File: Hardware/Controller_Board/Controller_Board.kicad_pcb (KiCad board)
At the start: 2 copper layers, 155 parts, among them Q1 DMN2400UFB-7, SW1 Reset, U1 TPS82084, U10 FT232H, U11 93LC56B, U2 LT8645S, U3 TPS82084, U4 TPS82084, U5 XT30, U6 XC7A35T-CPG236, U7 IS25LP256D, U8 FT232H, U9 93LC56B, Y1 12MHz, Y2 12MHz

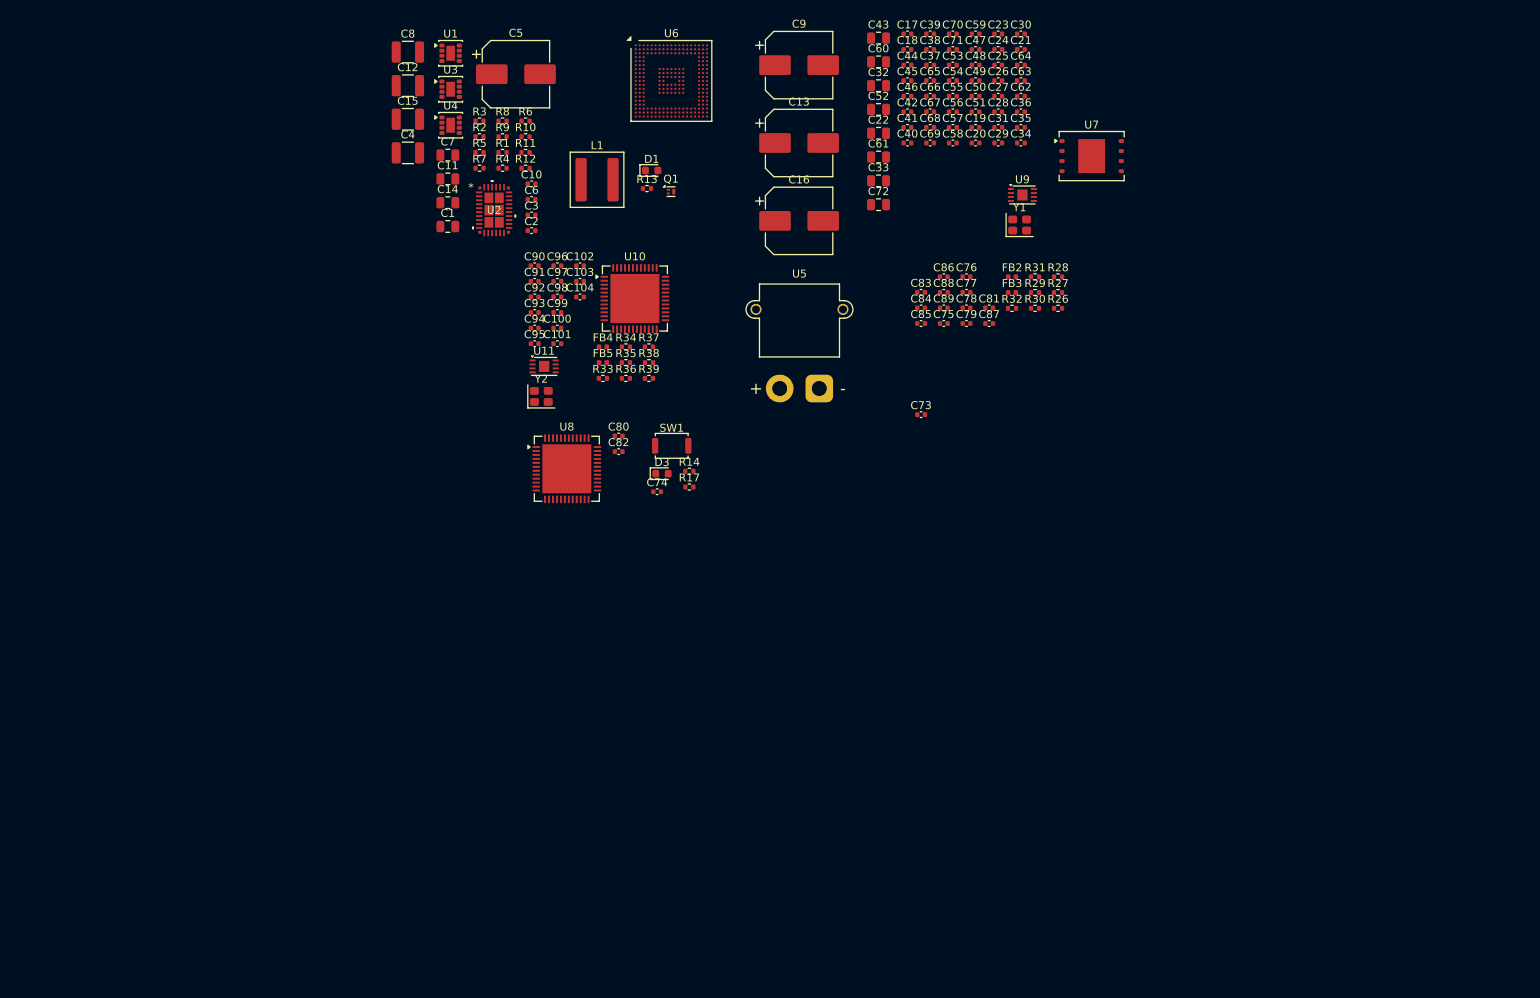
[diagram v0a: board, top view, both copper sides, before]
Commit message: Updated the schematic design - Fix the XC7A35T-CPG236 outline issue
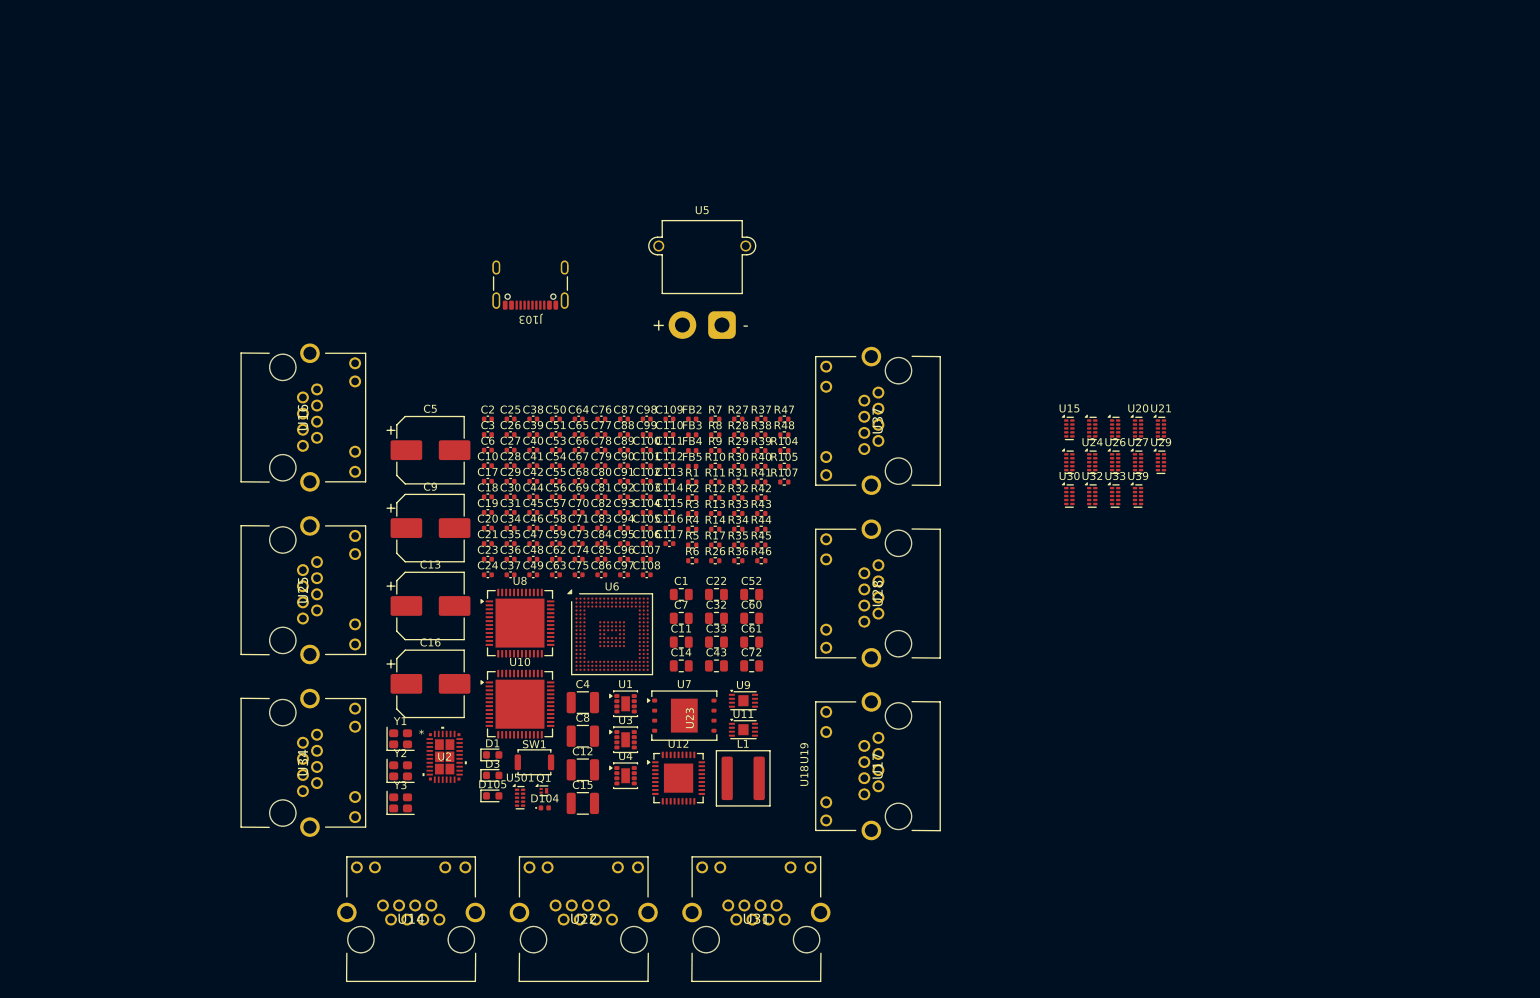
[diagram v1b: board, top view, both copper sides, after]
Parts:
- added C105: 10p, Capacitor_SMD:C_0402_1005Metric, F.Cu at (132.7, 94.0)
- added C106: 10p, Capacitor_SMD:C_0402_1005Metric, F.Cu at (132.7, 95.9)
- added C107: 4u7, Capacitor_SMD:C_0402_1005Metric, F.Cu at (132.7, 97.9)
- added C108: 100n, Capacitor_SMD:C_0402_1005Metric, F.Cu at (132.7, 99.9)
- added C109: 100n, Capacitor_SMD:C_0402_1005Metric, F.Cu at (135.6, 80.2)
- added C110: 100n, Capacitor_SMD:C_0402_1005Metric, F.Cu at (135.6, 82.1)
- added C111: 100n, Capacitor_SMD:C_0402_1005Metric, F.Cu at (135.6, 84.1)
- added C112: 100n, Capacitor_SMD:C_0402_1005Metric, F.Cu at (135.6, 86.1)
- added C113: 100n, Capacitor_SMD:C_0402_1005Metric, F.Cu at (135.6, 88.0)
- added C114: 10n, Capacitor_SMD:C_0402_1005Metric, F.Cu at (135.6, 90.0)
- added C115: 100n, Capacitor_SMD:C_0402_1005Metric, F.Cu at (135.6, 92.0)
- added C116: 10n, Capacitor_SMD:C_0402_1005Metric, F.Cu at (135.6, 94.0)
- added C117: 100n, Capacitor_SMD:C_0402_1005Metric, F.Cu at (135.6, 95.9)
- added D104: TVS, Diode_SMD:D_0402_1005Metric, F.Cu at (119.8, 129.3)
- added D105: LED, LED_SMD:LED_0603_1608Metric, F.Cu at (113.2, 127.8)
- added J103: USB_C_USB2.0, Connector_USB:USB_C_Receptacle_GCT_USB4105-xx-A_16P_TopMnt_Horizontal, F.Cu at (118.0, 62.1)
- added R104: 5k1, Resistor_SMD:R_0402_1005Metric, F.Cu at (150.1, 84.2)
- added R105: 5k1, Resistor_SMD:R_0402_1005Metric, F.Cu at (150.1, 86.1)
- added R107: 1k, Resistor_SMD:R_0402_1005Metric, F.Cu at (150.1, 88.1)
- added R40: 22R, Resistor_SMD:R_0402_1005Metric, F.Cu at (147.2, 86.1)
- added R41: 12k, Resistor_SMD:R_0402_1005Metric, F.Cu at (147.2, 88.1)
- added R42: 100k, Resistor_SMD:R_0402_1005Metric, F.Cu at (147.2, 90.1)
- added R43: 100k, Resistor_SMD:R_0402_1005Metric, F.Cu at (147.2, 92.1)
- added R44: 100k, Resistor_SMD:R_0402_1005Metric, F.Cu at (147.2, 94.1)
- added R45: 100k, Resistor_SMD:R_0402_1005Metric, F.Cu at (147.2, 96.1)
- added R46: 100k, Resistor_SMD:R_0402_1005Metric, F.Cu at (147.2, 98.1)
- added R47: 100k, Resistor_SMD:R_0402_1005Metric, F.Cu at (150.1, 80.2)
- added R48: 1k, Resistor_SMD:R_0402_1005Metric, F.Cu at (150.1, 82.2)
- added U12: USB2512B, Package_DFN_QFN:QFN-36-1EP_6x6mm_P0.5mm_EP3.7x3.7mm, F.Cu at (136.7, 125.6)
- added U14: RJ45, Custom_VoxLink_Footprints:TE_RJ45, F.Cu at (102.9, 146.0)
- added U15: TPD4E02B04, Package_SON:USON-10_2.5x1.0mm_P0.5mm, F.Cu at (186.1, 81.3)
- added U16: RJ45, Custom_VoxLink_Footprints:TE_RJ45, F.Cu at (86.7, 80.0)
- added U17: RJ45, Custom_VoxLink_Footprints:TE_RJ45, F.Cu at (164.5, 124.1)
- added U18: TPD4E02B04, Package_SON:USON-10_2.5x1.0mm_P0.5mm, F.Cu at (189.0, 81.3)
- added U19: TPD4E02B04, Package_SON:USON-10_2.5x1.0mm_P0.5mm, F.Cu at (191.9, 81.3)
- added U20: TPD4E02B04, Package_SON:USON-10_2.5x1.0mm_P0.5mm, F.Cu at (194.8, 81.3)
- added U21: TPD4E02B04, Package_SON:USON-10_2.5x1.0mm_P0.5mm, F.Cu at (197.7, 81.3)
- added U22: RJ45, Custom_VoxLink_Footprints:TE_RJ45, F.Cu at (124.7, 146.0)
- added U23: TPD4E02B04, Package_SON:USON-10_2.5x1.0mm_P0.5mm, F.Cu at (186.1, 85.6)
- added U24: TPD4E02B04, Package_SON:USON-10_2.5x1.0mm_P0.5mm, F.Cu at (189.0, 85.6)
- added U25: RJ45, Custom_VoxLink_Footprints:TE_RJ45, F.Cu at (86.7, 101.8)
- added U26: TPD4E02B04, Package_SON:USON-10_2.5x1.0mm_P0.5mm, F.Cu at (191.9, 85.6)
- added U27: TPD4E02B04, Package_SON:USON-10_2.5x1.0mm_P0.5mm, F.Cu at (194.8, 85.6)
- added U28: RJ45, Custom_VoxLink_Footprints:TE_RJ45, F.Cu at (164.5, 102.2)
- added U29: TPD4E02B04, Package_SON:USON-10_2.5x1.0mm_P0.5mm, F.Cu at (197.7, 85.6)
- added U30: TPD4E02B04, Package_SON:USON-10_2.5x1.0mm_P0.5mm, F.Cu at (186.1, 89.9)
- added U31: RJ45, Custom_VoxLink_Footprints:TE_RJ45, F.Cu at (146.6, 146.0)
- added U32: TPD4E02B04, Package_SON:USON-10_2.5x1.0mm_P0.5mm, F.Cu at (189.0, 89.9)
- added U33: TPD4E02B04, Package_SON:USON-10_2.5x1.0mm_P0.5mm, F.Cu at (191.9, 89.9)
- added U34: RJ45, Custom_VoxLink_Footprints:TE_RJ45, F.Cu at (86.7, 123.6)
- added U37: RJ45, Custom_VoxLink_Footprints:TE_RJ45, F.Cu at (164.5, 80.4)
- added U39: TPD4E02B04, Package_SON:USON-10_2.5x1.0mm_P0.5mm, F.Cu at (194.8, 89.9)
- added U501: TPD4E02B04, Package_SON:USON-10_2.5x1.0mm_P0.5mm, F.Cu at (116.7, 128.0)
- added Y3: 24MHz, Crystal:Crystal_SMD_2520-4Pin_2.5x2.0mm, F.Cu at (101.5, 128.7)
- moved Y1 101.7 mm to (101.5, 120.6)
- moved C23 92.6 mm to (112.6, 97.9)
- moved C24 92.6 mm to (112.6, 99.9)
- moved C21 91.9 mm to (112.6, 95.9)
- moved C15 89.3 mm to (124.6, 128.8)
- moved C12 89.3 mm to (124.6, 124.5)
- moved C8 89.3 mm to (124.6, 120.3)
- moved U7 87.5 mm to (137.4, 117.7)
- moved C30 87.1 mm to (115.5, 90.0)
- moved C36 85.8 mm to (115.5, 97.9)
- moved C63 85.8 mm to (121.2, 99.9)
- moved U1 85.2 mm to (130.0, 116.2)
- moved U3 85.2 mm to (130.0, 120.7)
- moved U4 85.2 mm to (130.0, 125.3)
- moved C47 83.9 mm to (118.3, 95.9)
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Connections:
- U10 pad 6: FTDI_USB_D- -> SERIAL_D-
- U10 pad 7: FTDI_USB_D+ -> SERIAL_D+
- U8 pad 6: FTDI_USB_D- -> JTAG_D-
- U8 pad 7: FTDI_USB_D+ -> JTAG_D+

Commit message: Finished schematic design - preparation for review
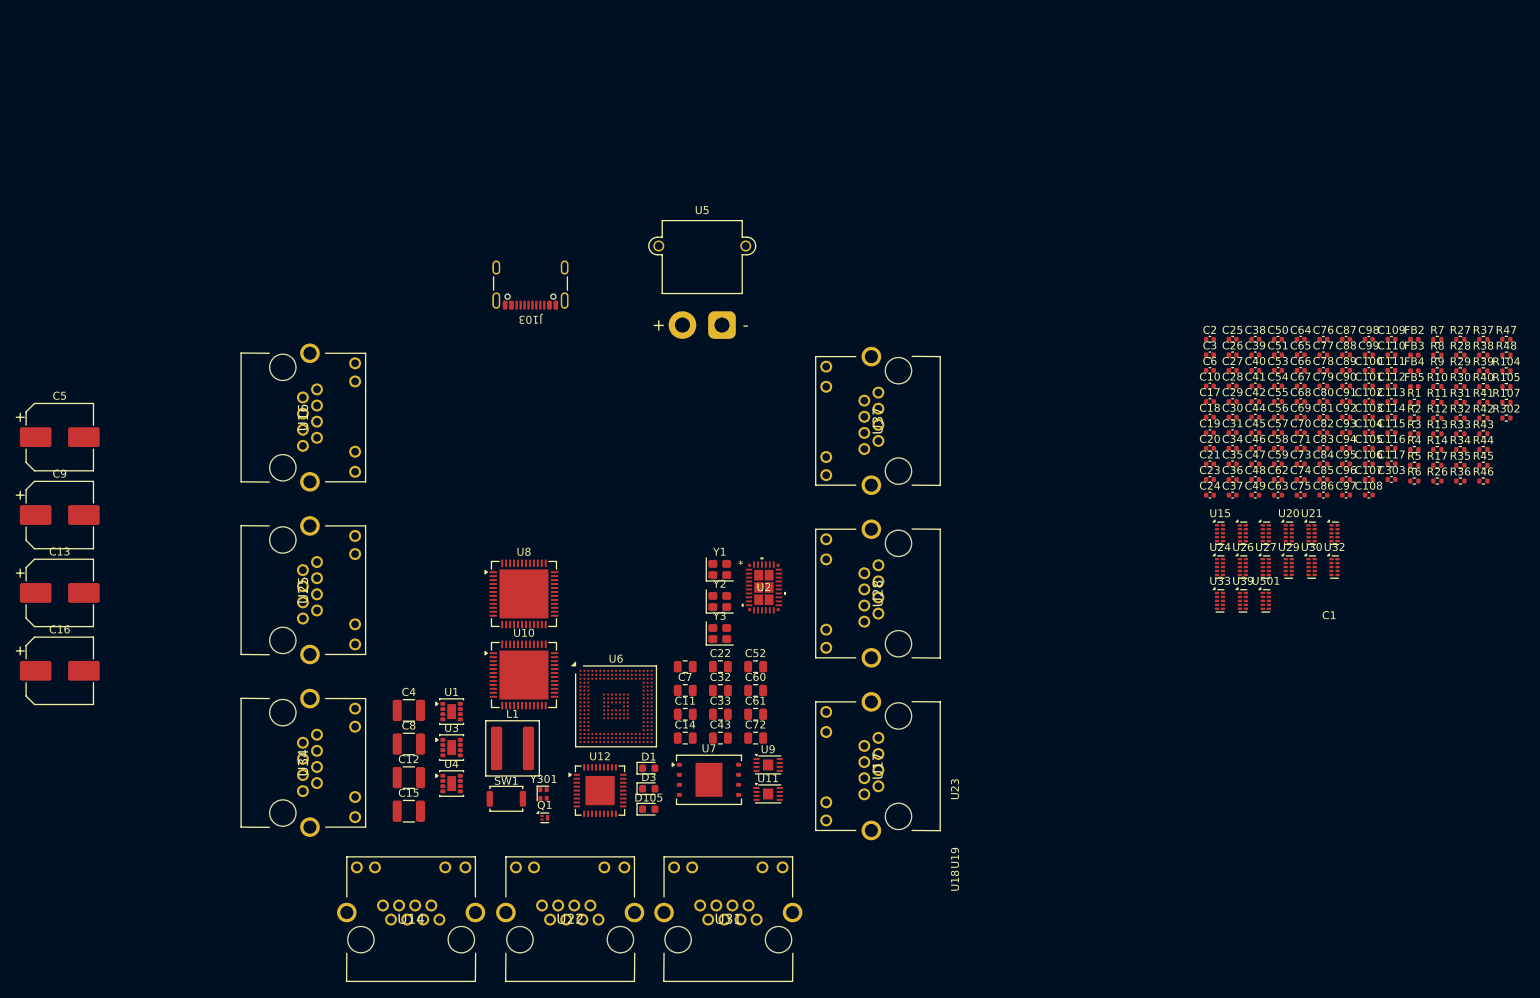
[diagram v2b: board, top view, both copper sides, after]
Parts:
- removed D104: TVS, Diode_SMD:D_0402_1005Metric
- added C303: 100n, Capacitor_SMD:C_0402_1005Metric, F.Cu at (226.9, 87.8)
- added R302: 22R, Resistor_SMD:R_0402_1005Metric, F.Cu at (241.4, 80.0)
- added Y301: 12MHz, Oscillator:Oscillator_SMD_Abracon_ASCO-4Pin_1.6x1.2mm, F.Cu at (119.6, 127.6)
- moved U501 97.5 mm to (211.0, 103.2)
- moved R27 91.9 mm to (235.6, 70.1)
- moved R28 91.9 mm to (235.6, 72.1)
- moved R29 91.9 mm to (235.6, 74.1)
- moved R30 91.9 mm to (235.6, 76.1)
- moved R31 91.9 mm to (235.6, 78.0)
- moved R32 91.9 mm to (235.6, 80.0)
- moved R33 91.9 mm to (235.6, 82.0)
- moved R34 91.9 mm to (235.6, 84.0)
- moved R35 91.9 mm to (235.6, 86.0)
- moved R36 91.9 mm to (235.6, 88.0)
- moved R37 91.9 mm to (238.5, 70.1)
- moved R38 91.9 mm to (238.5, 72.1)
- moved R39 91.9 mm to (238.5, 74.1)
- moved R40 91.9 mm to (238.5, 76.1)
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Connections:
- U14 pad 1: Net-(U14-RX) -> /Connectivity/P1_RX_P
- U14 pad 2: Net-(U14-~{RX}) -> /Connectivity/P1_RX_N
- U14 pad 4: Net-(U14-CLK) -> /Connectivity/P1_CLK_P
- U14 pad 5: Net-(U14-~{CLK}) -> /Connectivity/P1_CLK_N
- U14 pad 7: Net-(U14-~{TX}) -> /Connectivity/P1_TX_N
- U14 pad 8: Net-(U14-TX) -> /Connectivity/P1_TX_P
- U15 pad 1: Net-(U14-RX) -> /Connectivity/P1_RX_P
- U15 pad 10: unconnected-(U15-NC-Pad10) -> /Connectivity/P1_RX_P
- U15 pad 2: Net-(U14-~{RX}) -> /Connectivity/P1_RX_N
- U15 pad 4: Net-(U16-CLK) -> /Connectivity/P2_CLK_P
- U15 pad 5: Net-(U16-~{CLK}) -> /Connectivity/P2_CLK_N
- U15 pad 6: unconnected-(U15-NC-Pad6) -> /Connectivity/P2_CLK_N
- U15 pad 7: unconnected-(U15-NC-Pad7) -> /Connectivity/P2_CLK_P
- U15 pad 9: unconnected-(U15-NC-Pad9) -> /Connectivity/P1_RX_N
- U16 pad 1: Net-(U16-RX) -> /Connectivity/P2_RX_P
- U16 pad 2: Net-(U16-~{RX}) -> /Connectivity/P2_RX_N
- U16 pad 4: Net-(U16-CLK) -> /Connectivity/P2_CLK_P
- U16 pad 5: Net-(U16-~{CLK}) -> /Connectivity/P2_CLK_N
- U16 pad 7: Net-(U16-~{TX}) -> /Connectivity/P2_TX_N
- U16 pad 8: Net-(U16-TX) -> /Connectivity/P2_TX_P
- U17 pad 1: Net-(U17-RX) -> /Connectivity/P3_RX_P
- U17 pad 2: Net-(U17-~{RX}) -> /Connectivity/P3_RX_N
- U17 pad 4: Net-(U17-CLK) -> /Connectivity/P3_CLK_P
- U17 pad 5: Net-(U17-~{CLK}) -> /Connectivity/P3_CLK_N
- U17 pad 7: Net-(U17-~{TX}) -> /Connectivity/P3_TX_N
- U17 pad 8: Net-(U17-TX) -> /Connectivity/P3_TX_P
- U18 pad 1: Net-(U17-~{TX}) -> /Connectivity/P3_TX_N
- U18 pad 10: unconnected-(U18-NC-Pad10) -> /Connectivity/P3_TX_N
- U18 pad 2: Net-(U17-TX) -> /Connectivity/P3_TX_P
- U18 pad 4: Net-(U17-~{CLK}) -> /Connectivity/P3_CLK_N
- U18 pad 5: Net-(U17-CLK) -> /Connectivity/P3_CLK_P
- U18 pad 6: unconnected-(U18-NC-Pad6) -> /Connectivity/P3_CLK_P
- U18 pad 7: unconnected-(U18-NC-Pad7) -> /Connectivity/P3_CLK_N
- U18 pad 9: unconnected-(U18-NC-Pad9) -> /Connectivity/P3_TX_P
- U19 pad 4: Net-(U17-~{RX}) -> /Connectivity/P3_RX_N
- U19 pad 5: Net-(U17-RX) -> /Connectivity/P3_RX_P
- U19 pad 6: unconnected-(U19-NC-Pad6) -> /Connectivity/P3_RX_P
- U19 pad 7: unconnected-(U19-NC-Pad7) -> /Connectivity/P3_RX_N
- U20 pad 1: Net-(U16-~{RX}) -> /Connectivity/P2_RX_N
- U20 pad 10: unconnected-(U20-NC-Pad10) -> /Connectivity/P2_RX_N
- U20 pad 2: Net-(U16-RX) -> /Connectivity/P2_RX_P
- U20 pad 4: Net-(U16-~{TX}) -> /Connectivity/P2_TX_N
- U20 pad 5: Net-(U16-TX) -> /Connectivity/P2_TX_P
- U20 pad 6: unconnected-(U20-NC-Pad6) -> /Connectivity/P2_TX_P
- U20 pad 7: unconnected-(U20-NC-Pad7) -> /Connectivity/P2_TX_N
- U20 pad 9: unconnected-(U20-NC-Pad9) -> /Connectivity/P2_RX_P
- U21 pad 1: Net-(U37-~{TX}) -> /Connectivity/P9_TX_N
- U21 pad 10: unconnected-(U21-NC-Pad10) -> /Connectivity/P9_TX_N
- U21 pad 2: Net-(U37-TX) -> /Connectivity/P9_TX_P
- U21 pad 4: Net-(U37-~{CLK}) -> /Connectivity/P9_CLK_N
- U21 pad 5: Net-(U37-CLK) -> /Connectivity/P9_CLK_P
- U21 pad 6: unconnected-(U21-NC-Pad6) -> /Connectivity/P9_CLK_P
- U21 pad 7: unconnected-(U21-NC-Pad7) -> /Connectivity/P9_CLK_N
- U21 pad 9: unconnected-(U21-NC-Pad9) -> /Connectivity/P9_TX_P
- U22 pad 1: Net-(U22-RX) -> /Connectivity/P4_RX_P
- U22 pad 2: Net-(U22-~{RX}) -> /Connectivity/P4_RX_N
- U22 pad 4: Net-(U22-CLK) -> /Connectivity/P4_CLK_P
- U22 pad 5: Net-(U22-~{CLK}) -> /Connectivity/P4_CLK_N
- U22 pad 7: Net-(U22-~{TX}) -> /Connectivity/P4_TX_N
- U22 pad 8: Net-(U22-TX) -> /Connectivity/P4_TX_P
- U23 pad 1: Net-(U22-~{TX}) -> /Connectivity/P4_TX_N
- U23 pad 10: unconnected-(U23-NC-Pad10) -> /Connectivity/P4_TX_N
- U23 pad 2: Net-(U22-TX) -> /Connectivity/P4_TX_P
- U23 pad 4: Net-(U22-~{CLK}) -> /Connectivity/P4_CLK_N
- U23 pad 5: Net-(U22-CLK) -> /Connectivity/P4_CLK_P
- U23 pad 6: unconnected-(U23-NC-Pad6) -> /Connectivity/P4_CLK_P
- U23 pad 7: unconnected-(U23-NC-Pad7) -> /Connectivity/P4_CLK_N
- U23 pad 9: unconnected-(U23-NC-Pad9) -> /Connectivity/P4_TX_P
- U24 pad 1: Net-(U25-~{RX}) -> /Connectivity/P5_RX_N
- U24 pad 10: unconnected-(U24-NC-Pad10) -> /Connectivity/P5_RX_N
- U24 pad 2: Net-(U25-RX) -> /Connectivity/P5_RX_P
- U24 pad 4: Net-(U25-~{TX}) -> /Connectivity/P5_TX_N
- U24 pad 5: Net-(U25-TX) -> /Connectivity/P5_TX_P
- U24 pad 6: unconnected-(U24-NC-Pad6) -> /Connectivity/P5_TX_P
- U24 pad 7: unconnected-(U24-NC-Pad7) -> /Connectivity/P5_TX_N
- U24 pad 9: unconnected-(U24-NC-Pad9) -> /Connectivity/P5_RX_P
- U25 pad 1: Net-(U25-RX) -> /Connectivity/P5_RX_P
- U25 pad 2: Net-(U25-~{RX}) -> /Connectivity/P5_RX_N
- U25 pad 4: Net-(U25-CLK) -> /Connectivity/P5_CLK_P
- U25 pad 5: Net-(U25-~{CLK}) -> /Connectivity/P5_CLK_N
- U25 pad 7: Net-(U25-~{TX}) -> /Connectivity/P5_TX_N
- U25 pad 8: Net-(U25-TX) -> /Connectivity/P5_TX_P
- U26 pad 1: Net-(U34-~{RX}) -> /Connectivity/P8_RX_N
- U26 pad 10: unconnected-(U26-NC-Pad10) -> /Connectivity/P8_RX_N
- U26 pad 2: Net-(U34-RX) -> /Connectivity/P8_RX_P
- U26 pad 4: Net-(U34-~{TX}) -> /Connectivity/P8_TX_N
- U26 pad 5: Net-(U34-TX) -> /Connectivity/P8_TX_P
- U26 pad 6: unconnected-(U26-NC-Pad6) -> /Connectivity/P8_TX_P
- U26 pad 7: unconnected-(U26-NC-Pad7) -> /Connectivity/P8_TX_N
- U26 pad 9: unconnected-(U26-NC-Pad9) -> /Connectivity/P8_RX_P
- U27 pad 1: Net-(U22-RX) -> /Connectivity/P4_RX_P
- U27 pad 10: unconnected-(U27-NC-Pad10) -> /Connectivity/P4_RX_P
- U27 pad 2: Net-(U22-~{RX}) -> /Connectivity/P4_RX_N
- U27 pad 4: Net-(U25-CLK) -> /Connectivity/P5_CLK_P
- U27 pad 5: Net-(U25-~{CLK}) -> /Connectivity/P5_CLK_N
- U27 pad 6: unconnected-(U27-NC-Pad6) -> /Connectivity/P5_CLK_N
- U27 pad 7: unconnected-(U27-NC-Pad7) -> /Connectivity/P5_CLK_P
- U27 pad 9: unconnected-(U27-NC-Pad9) -> /Connectivity/P4_RX_N
- U28 pad 1: Net-(U28-RX) -> /Connectivity/P6_RX_P
- U28 pad 2: Net-(U28-~{RX}) -> /Connectivity/P6_RX_N
- U28 pad 4: Net-(U28-CLK) -> /Connectivity/P6_CLK_P
- U28 pad 5: Net-(U28-~{CLK}) -> /Connectivity/P6_CLK_N
- U28 pad 7: Net-(U28-~{TX}) -> /Connectivity/P6_TX_N
- U28 pad 8: Net-(U28-TX) -> /Connectivity/P6_TX_P
- U29 pad 1: Net-(U28-~{TX}) -> /Connectivity/P6_TX_N
- U29 pad 10: unconnected-(U29-NC-Pad10) -> /Connectivity/P6_TX_N
- U29 pad 2: Net-(U28-TX) -> /Connectivity/P6_TX_P
- U29 pad 4: Net-(U28-~{CLK}) -> /Connectivity/P6_CLK_N
- U29 pad 5: Net-(U28-CLK) -> /Connectivity/P6_CLK_P
- U29 pad 6: unconnected-(U29-NC-Pad6) -> /Connectivity/P6_CLK_P
- U29 pad 7: unconnected-(U29-NC-Pad7) -> /Connectivity/P6_CLK_N
- U29 pad 9: unconnected-(U29-NC-Pad9) -> /Connectivity/P6_TX_P
- U30 pad 4: Net-(U28-~{RX}) -> /Connectivity/P6_RX_N
- U30 pad 5: Net-(U28-RX) -> /Connectivity/P6_RX_P
- U30 pad 6: unconnected-(U30-NC-Pad6) -> /Connectivity/P6_RX_P
- U30 pad 7: unconnected-(U30-NC-Pad7) -> /Connectivity/P6_RX_N
- U31 pad 1: Net-(U31-RX) -> /Connectivity/P7_RX_P
- U31 pad 2: Net-(U31-~{RX}) -> /Connectivity/P7_RX_N
- U31 pad 4: Net-(U31-CLK) -> /Connectivity/P7_CLK_P
- U31 pad 5: Net-(U31-~{CLK}) -> /Connectivity/P7_CLK_N
- U31 pad 7: Net-(U31-~{TX}) -> /Connectivity/P7_TX_N
- U31 pad 8: Net-(U31-TX) -> /Connectivity/P7_TX_P
- U32 pad 1: Net-(U31-~{TX}) -> /Connectivity/P7_TX_N
- U32 pad 10: unconnected-(U32-NC-Pad10) -> /Connectivity/P7_TX_N
- U32 pad 2: Net-(U31-TX) -> /Connectivity/P7_TX_P
- U32 pad 4: Net-(U31-~{CLK}) -> /Connectivity/P7_CLK_N
- U32 pad 5: Net-(U31-CLK) -> /Connectivity/P7_CLK_P
- U32 pad 6: unconnected-(U32-NC-Pad6) -> /Connectivity/P7_CLK_P
- U32 pad 7: unconnected-(U32-NC-Pad7) -> /Connectivity/P7_CLK_N
- U32 pad 9: unconnected-(U32-NC-Pad9) -> /Connectivity/P7_TX_P
- U33 pad 1: Net-(U31-RX) -> /Connectivity/P7_RX_P
- U33 pad 10: unconnected-(U33-NC-Pad10) -> /Connectivity/P7_RX_P
- U33 pad 2: Net-(U31-~{RX}) -> /Connectivity/P7_RX_N
- U33 pad 4: Net-(U34-CLK) -> /Connectivity/P8_CLK_P
- U33 pad 5: Net-(U34-~{CLK}) -> /Connectivity/P8_CLK_N
- U33 pad 6: unconnected-(U33-NC-Pad6) -> /Connectivity/P8_CLK_N
- U33 pad 7: unconnected-(U33-NC-Pad7) -> /Connectivity/P8_CLK_P
- U33 pad 9: unconnected-(U33-NC-Pad9) -> /Connectivity/P7_RX_N
- U34 pad 1: Net-(U34-RX) -> /Connectivity/P8_RX_P
- U34 pad 2: Net-(U34-~{RX}) -> /Connectivity/P8_RX_N
- U34 pad 4: Net-(U34-CLK) -> /Connectivity/P8_CLK_P
- U34 pad 5: Net-(U34-~{CLK}) -> /Connectivity/P8_CLK_N
- U34 pad 7: Net-(U34-~{TX}) -> /Connectivity/P8_TX_N
- U34 pad 8: Net-(U34-TX) -> /Connectivity/P8_TX_P
- U37 pad 1: Net-(U37-RX) -> /Connectivity/P9_RX_P
- U37 pad 2: Net-(U37-~{RX}) -> /Connectivity/P9_RX_N
- U37 pad 4: Net-(U37-CLK) -> /Connectivity/P9_CLK_P
- U37 pad 5: Net-(U37-~{CLK}) -> /Connectivity/P9_CLK_N
- U37 pad 7: Net-(U37-~{TX}) -> /Connectivity/P9_TX_N
- U37 pad 8: Net-(U37-TX) -> /Connectivity/P9_TX_P
- U39 pad 4: Net-(U37-~{RX}) -> /Connectivity/P9_RX_N
- U39 pad 5: Net-(U37-RX) -> /Connectivity/P9_RX_P
- U39 pad 6: unconnected-(U39-NC-Pad6) -> /Connectivity/P9_RX_P
- U39 pad 7: unconnected-(U39-NC-Pad7) -> /Connectivity/P9_RX_N
- U501 pad 1: Net-(U14-~{TX}) -> /Connectivity/P1_TX_N
- U501 pad 10: unconnected-(U501-NC-Pad10) -> /Connectivity/P1_TX_N
- U501 pad 2: Net-(U14-TX) -> /Connectivity/P1_TX_P
- U501 pad 4: Net-(U14-~{CLK}) -> /Connectivity/P1_CLK_N
- U501 pad 5: Net-(U14-CLK) -> /Connectivity/P1_CLK_P
- U501 pad 6: unconnected-(U501-NC-Pad6) -> /Connectivity/P1_CLK_P
- U501 pad 7: unconnected-(U501-NC-Pad7) -> /Connectivity/P1_CLK_N
- U501 pad 9: unconnected-(U501-NC-Pad9) -> /Connectivity/P1_TX_P
- U6 pad A10: (no net) -> unconnected-(U6C-MGTREFCLK1N_216-PadA10)
- U6 pad A2: (no net) -> unconnected-(U6C-MGTPTXN1_216-PadA2)
- U6 pad A4: (no net) -> GND
- U6 pad A6: (no net) -> GND
- U6 pad A8: (no net) -> unconnected-(U6C-MGTREFCLK0N_216-PadA8)
- U6 pad B10: (no net) -> unconnected-(U6C-MGTREFCLK1P_216-PadB10)
- U6 pad B2: (no net) -> unconnected-(U6C-MGTPTXP1_216-PadB2)
- U6 pad B4: (no net) -> GND
- U6 pad B6: (no net) -> GND
- U6 pad B8: (no net) -> unconnected-(U6C-MGTREFCLK0P_216-PadB8)
- U6 pad C7: (no net) -> GND
- U6 pad D1: (no net) -> unconnected-(U6C-MGTPTXN0_216-PadD1)
- U6 pad D2: (no net) -> unconnected-(U6C-MGTPTXP0_216-PadD2)
- U6 pad E18: (no net) -> /Connectivity/P1_CLK_P
- U6 pad E19: (no net) -> /Connectivity/P1_CLK_N
- U6 pad G17: (no net) -> /Connectivity/P1_RX_N
- U6 pad G19: (no net) -> /Connectivity/P1_TX_N
- U6 pad H17: (no net) -> /Connectivity/P1_RX_P
- U6 pad H19: (no net) -> /Connectivity/P1_TX_P
- U6 pad J17: (no net) -> /Connectivity/P2_CLK_P
- U6 pad J18: (no net) -> /Connectivity/P2_CLK_N
- U6 pad K17: (no net) -> /Connectivity/P3_RX_N
- U6 pad K18: (no net) -> /Connectivity/P2_TX_N
- U6 pad L17: (no net) -> /Connectivity/P3_RX_P
- U6 pad L18: (no net) -> /Connectivity/P2_TX_P
- U6 pad M18: (no net) -> /Connectivity/P3_TX_P
- U6 pad M19: (no net) -> /Connectivity/P3_TX_N
- U6 pad N17: (no net) -> /Connectivity/P4_CLK_P
- U6 pad N18: (no net) -> /Connectivity/P2_RX_P
- U6 pad N19: (no net) -> /Connectivity/P2_RX_N
- U6 pad P17: (no net) -> /Connectivity/P4_CLK_N
- U6 pad P18: (no net) -> /Connectivity/P4_TX_P
- U6 pad P19: (no net) -> /Connectivity/P3_CLK_P
- U6 pad R18: (no net) -> /Connectivity/P4_TX_N
- U6 pad R19: (no net) -> /Connectivity/P3_CLK_N
- U6 pad T17: (no net) -> /Connectivity/P5_TX_P
- U6 pad T18: (no net) -> /Connectivity/P5_TX_N
- U6 pad U15: (no net) -> /Connectivity/P7_TX_P
- U6 pad U16: (no net) -> /Connectivity/P7_TX_N
- U6 pad U17: (no net) -> /Connectivity/P5_RX_P
- U6 pad U18: (no net) -> /Connectivity/P5_RX_N
- U6 pad U19: (no net) -> /Connectivity/P4_RX_P
- U6 pad V13: (no net) -> /Connectivity/P7_RX_P
- U6 pad V14: (no net) -> /Connectivity/P7_RX_N
- U6 pad V15: (no net) -> /Connectivity/P6_RX_P
- U6 pad V16: (no net) -> /Connectivity/P6_CLK_P
- U6 pad V17: (no net) -> /Connectivity/P6_CLK_N
- U6 pad V19: (no net) -> /Connectivity/P4_RX_N
- U6 pad W13: (no net) -> /Connectivity/P7_CLK_P
- U6 pad W14: (no net) -> /Connectivity/P7_CLK_N
- U6 pad W15: (no net) -> /Connectivity/P6_RX_N
- U6 pad W16: (no net) -> /Connectivity/P6_TX_P
- U6 pad W17: (no net) -> /Connectivity/P6_TX_N
- U6 pad W18: (no net) -> /Connectivity/P5_CLK_P
- U6 pad W19: (no net) -> /Connectivity/P5_CLK_N
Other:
- copper layers 2 -> 8
